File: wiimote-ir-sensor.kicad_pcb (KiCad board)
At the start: 2 copper layers, 13.5 x 18 mm, 10 parts, among them J1 Conn_01x04_Pin, U2 AP2112-3.3V, X1 X1G004451000300

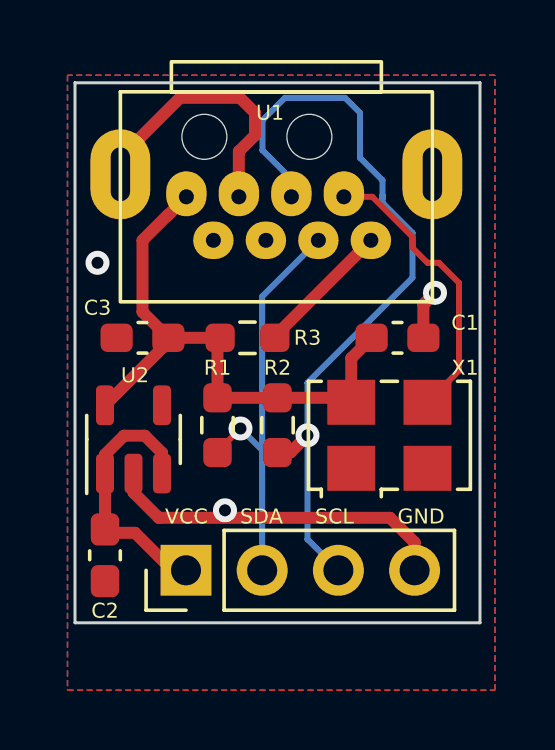
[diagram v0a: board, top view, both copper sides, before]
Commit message: First usable revision
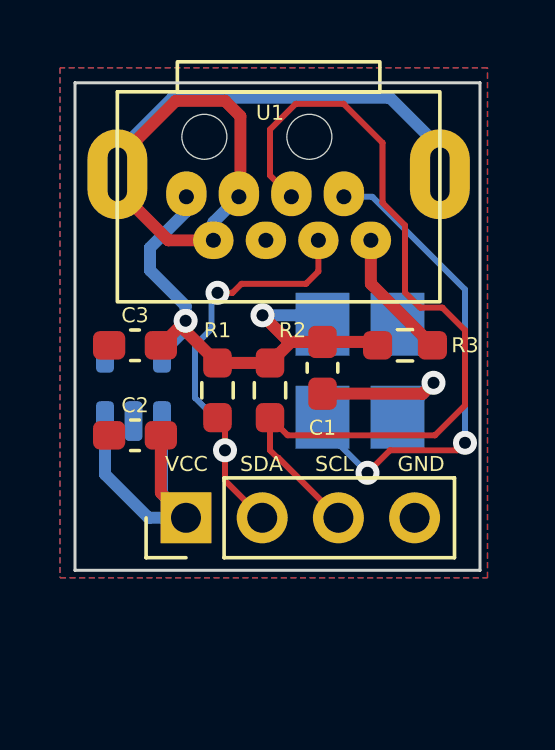
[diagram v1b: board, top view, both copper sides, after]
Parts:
- U2: moved to B.Cu
- X1: value X1G004451000300 -> SG3225CAN 24.0000M-TJGA3; footprint Oscillator:Oscillator_SMD_SeikoEpson_SG8002LB-4Pin_5.0x3.2mm -> Oscillator:Oscillator_SMD_SeikoEpson_SG8002CE-4Pin_3.2x2.5mm_HandSoldering; moved to B.Cu
- moved R3 5.26 mm to (159.8, 86.8)
- moved C2 4.12 mm to (150.8, 89.8), turned to 180 degrees
- moved C1 2.69 mm to (157.0, 87.5), turned to -90 degrees
- moved X1 2.36 mm to (158.2, 87.6), turned to -90 degrees
- moved J1 1.75 mm to (152.4, 92.5)
- moved U2 1.75 mm to (150.7, 88.1)
- moved R2 1.19 mm to (155.2, 88.2)
- moved R1 1.16 mm to (153.5, 88.2)
- moved C3 0.35 mm to (150.8, 86.8)
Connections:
- X1 pad 1: GND -> unconnected-(X1-~{ST}-Pad1)
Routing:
- net GND: track 21.8 -> 30.5 mm, vias 3 -> 1
- net /CLK: track 9.65 -> 17.2 mm, vias 0 -> 2
- net /SCL: track 25.3 -> 29.0 mm, vias 1 -> 0
- net +5V: track 8.24 -> 11.7 mm
- net Net-(U1-RESET): track 4.53 -> 4.00 mm
- net +3.3V: track 19.0 -> 18.6 mm, vias 0 -> 2
- net /SDA: track 13.9 -> 14.3 mm, vias 1 -> 2
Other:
- board size 13.5 x 18 mm -> 13.5 x 16.2 mm
